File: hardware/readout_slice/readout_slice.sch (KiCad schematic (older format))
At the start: 4 parts

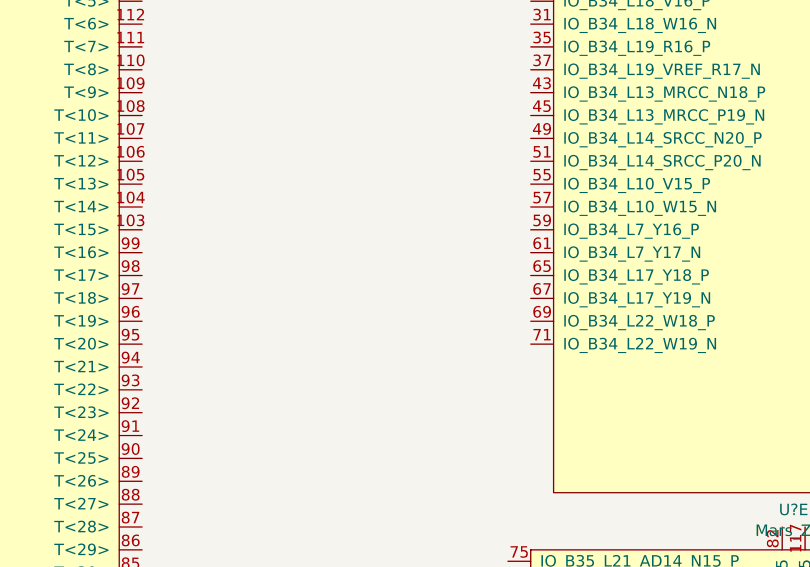
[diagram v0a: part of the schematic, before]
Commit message: working on readount_slice
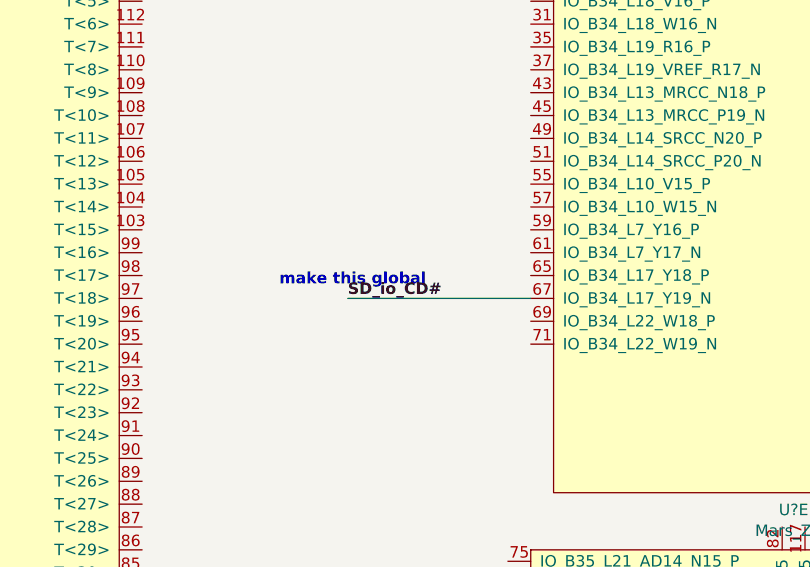
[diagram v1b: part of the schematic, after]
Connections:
- net SD_io_CD#: now reaches U?.67 (IO_B34_L17_Y19_N)
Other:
- note added: "make this global"
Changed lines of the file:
@@
 F1 "FPGA.sch" 50
 $EndSheet
+Wire Wire Line
+	6100 2800 5300 2800
+Text Notes 5000 2750 0    50   ~ 10
+make this global
+Text Label 5300 2800 0    50   ~ 10
+SD_io_CD#
 $EndSCHEMATC

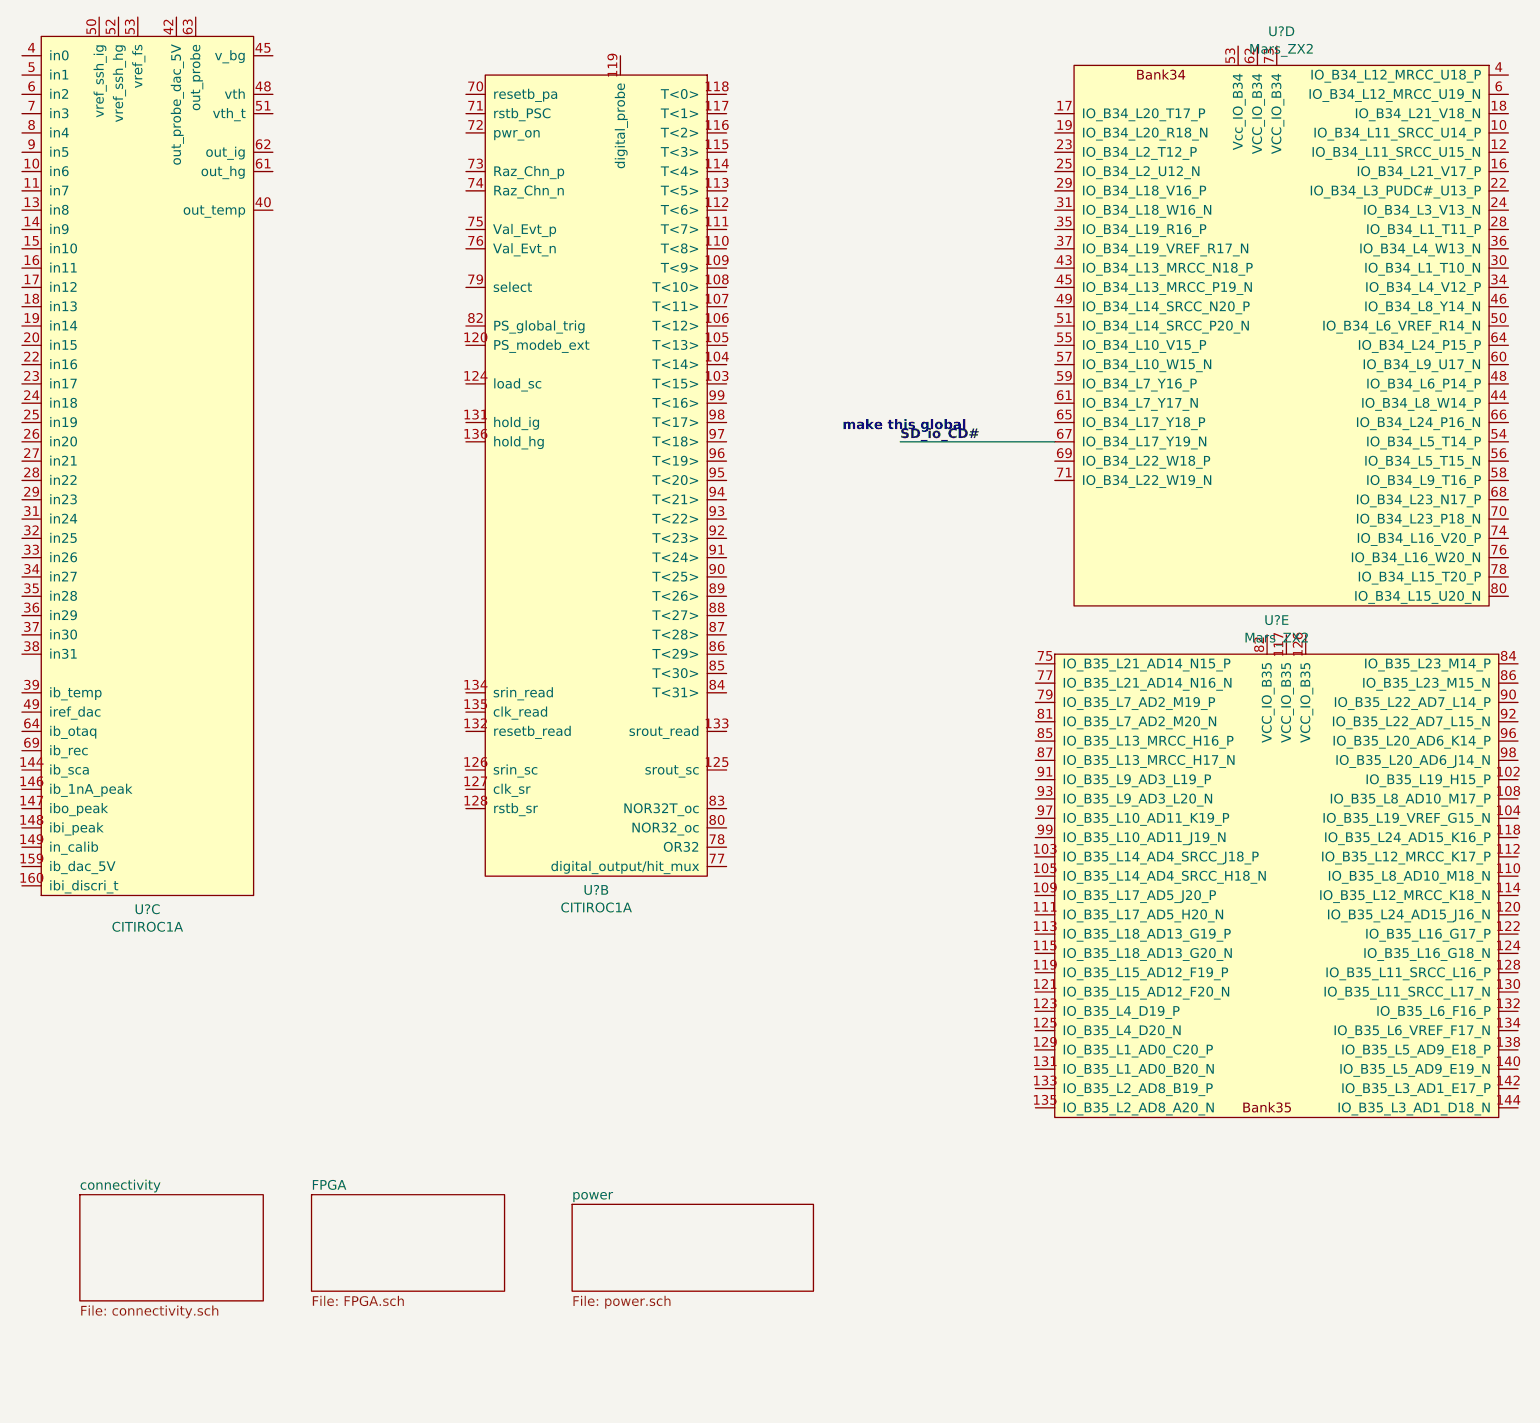
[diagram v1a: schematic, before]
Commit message: more work on readout_slice
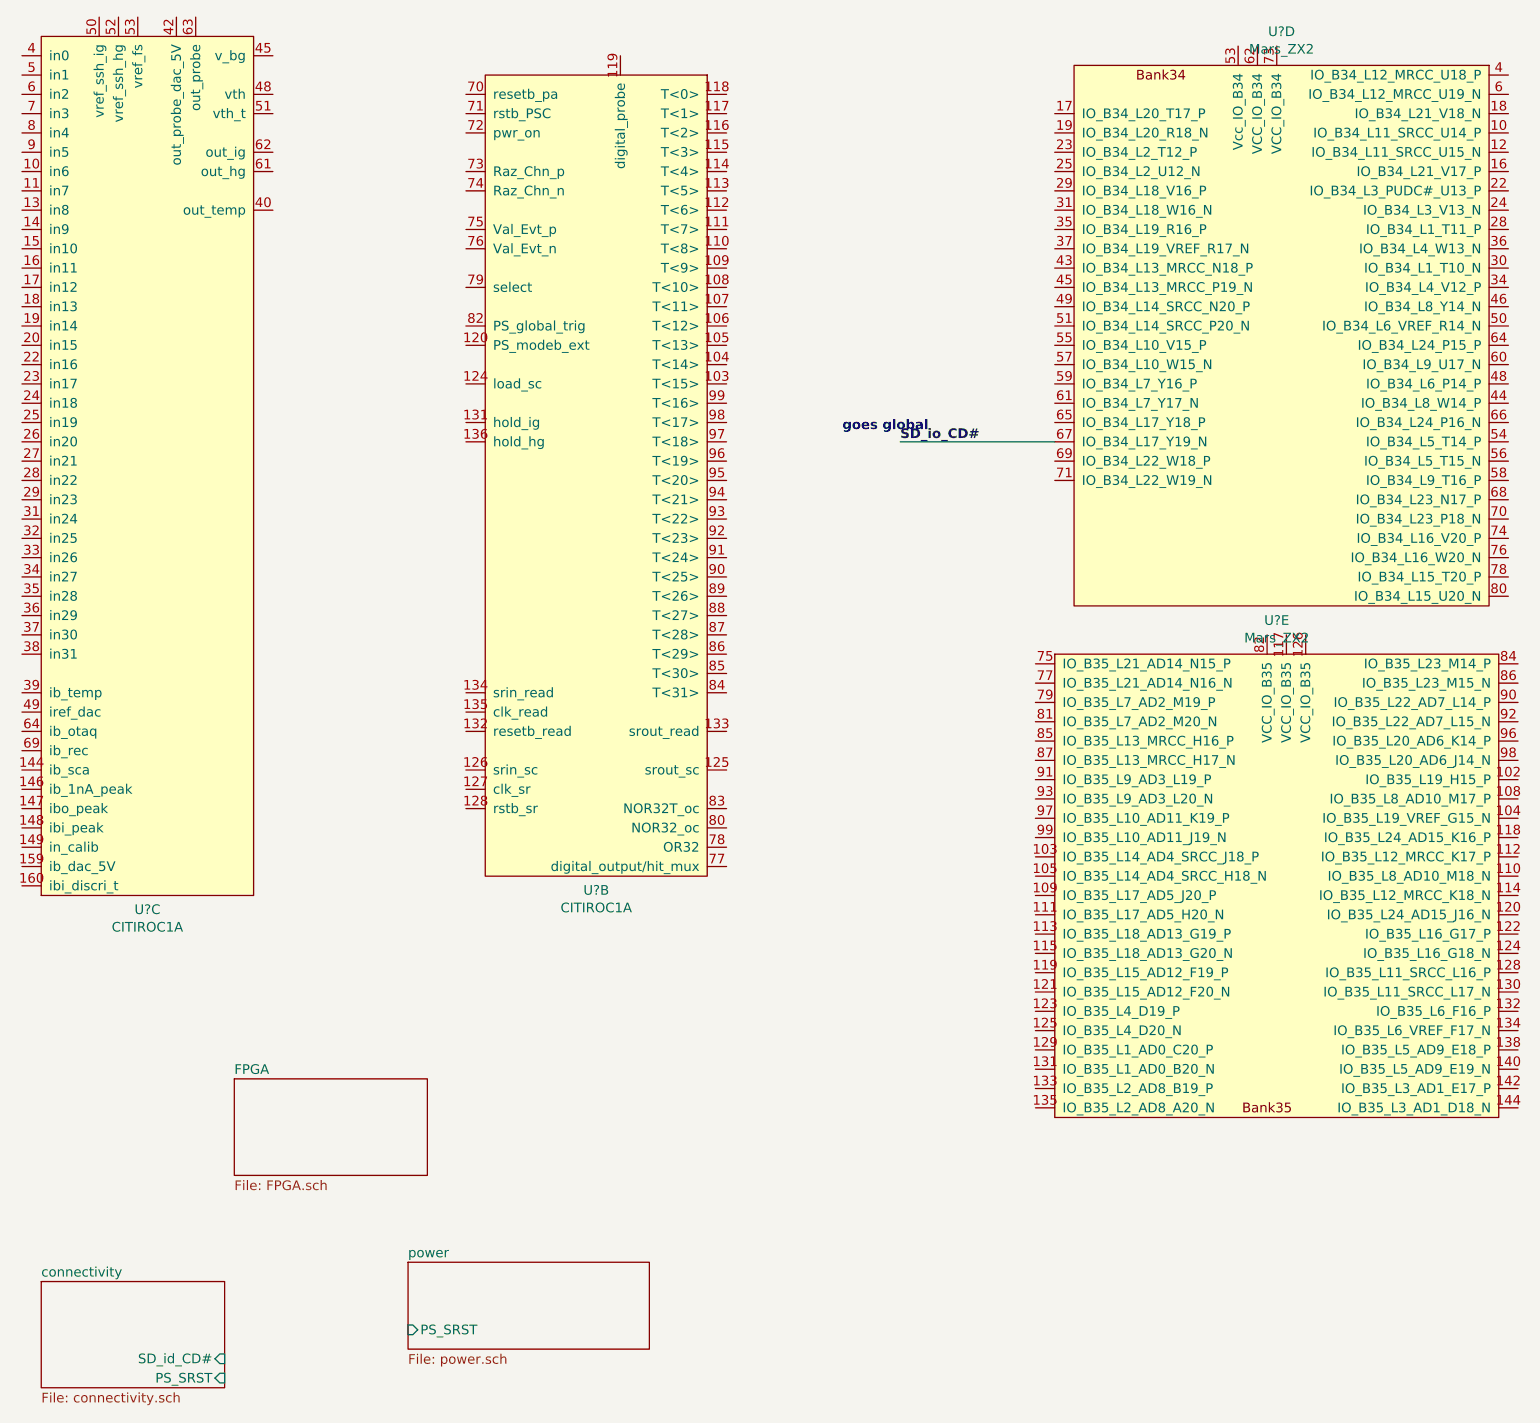
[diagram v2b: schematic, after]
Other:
- note added: "goes global"
- note removed: "make this global"
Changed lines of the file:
@@
 $EndComp
 $Sheet
-S 3600 6750 1250 450
+S 2750 7050 1250 450
 U 603D0C5A
 F0 "power" 50
 F1 "power.sch" 50
+F2 "PS_SRST" I L 2750 7400 50
 $EndSheet
 $Comp
@@
 $EndComp
 $Sheet
-S 1050 6700 950  550
+S 850  7150 950  550
 U 608B2FC0
 F0 "connectivity" 50
 F1 "connectivity.sch" 50
+F2 "PS_SRST" I R 1800 7650 50
+F3 "SD_id_CD#" I R 1800 7550 50
 $EndSheet
 $Comp
@@
 $EndComp
 $Sheet
-S 2250 6700 1000 500
+S 1850 6100 1000 500
 U 605605C8
 F0 "FPGA" 50
@@
 	6100 2800 5300 2800
 Text Notes 5000 2750 0    50   ~ 10
-make this global
+goes global
 Text Label 5300 2800 0    50   ~ 10
 SD_io_CD#
